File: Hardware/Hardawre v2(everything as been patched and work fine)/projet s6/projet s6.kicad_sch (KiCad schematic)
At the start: 23 parts, among them SW5 RSTBTN, SW6 Int, SW7 boot, U1 STM32L432KCUx, U2 LTC4065AEDC, U3 LDLN022PU33R

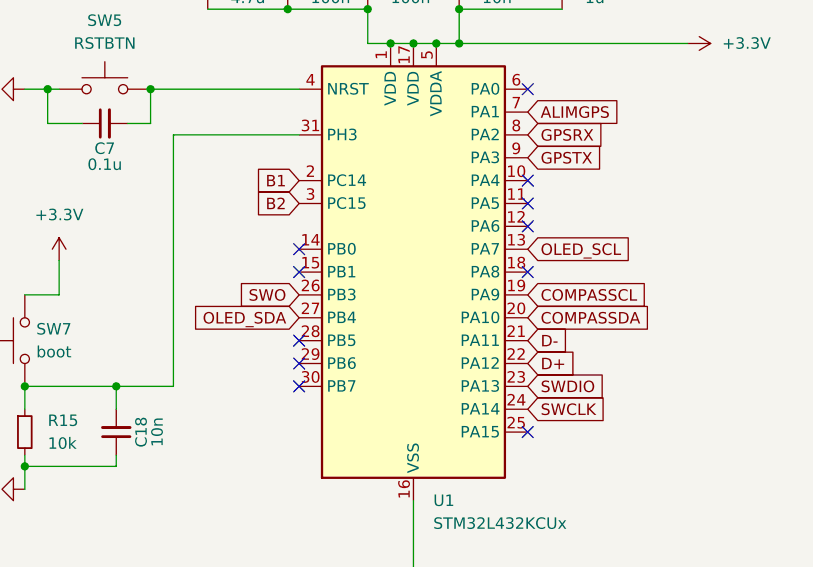
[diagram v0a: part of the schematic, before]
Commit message: gr
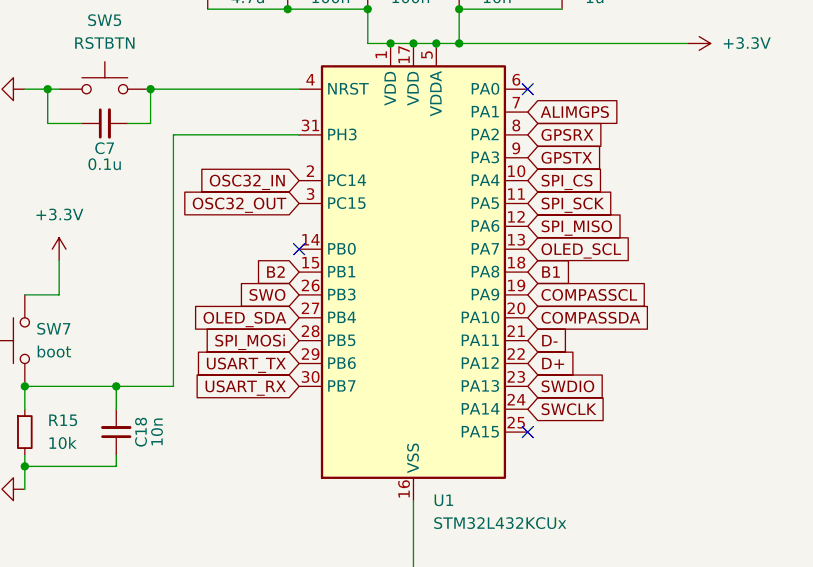
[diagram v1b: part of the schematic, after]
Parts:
- SW5, SW7: footprint SW_KXT3:SW_KXT3 -> KXT3:SW_KXT3
- SW6: footprint SW_PCM:SW_PCM -> PCM:SW_PCM
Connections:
- net B1: now also U1.18 (PA8); no longer U1.2 (PC14)
- net B2: now also U1.15 (PB1); no longer U1.3 (PC15)
- net SPI_CS: now reaches U1.10 (PA4)
- net SPI_SCK: now reaches U1.11 (PA5)
- net SPI_MISO: now reaches U1.12 (PA6)
- net SPI_MOSi: now reaches U1.28 (PB5)
- net USART_TX: now reaches U1.29 (PB6)
- net USART_RX: now reaches U1.30 (PB7)
- new net OSC32_IN: U1.2 (PC14)
- new net OSC32_OUT: U1.3 (PC15)
- no-connect marks 11 -> 3
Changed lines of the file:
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@@
 	)
 	(no_connect
-		(at 233.68 80.01)
-	)
-	(no_connect
-		(at 208.28 95.25)
-	)
-	(no_connect
-		(at 233.68 85.09)
-	)
-	(no_connect
 		(at 233.68 102.87)
 	)
 	(no_connect
-		(at 233.68 74.93)
-	)
-	(no_connect
 		(at 233.68 64.77)
 	)
 	(no_connect
-		(at 208.28 92.71)
-	)
-	(no_connect
-		(at 208.28 97.79)
-	)
-	(no_connect
 		(at 208.28 82.55)
 	)
-	(no_connect
-		(at 208.28 85.09)
-	)
-	(no_connect
-		(at 233.68 77.47)
-	)
 	(wire
 		(pts
@@
 		)
 	)
+	(global_label "OSC32_OUT"
+		(shape input)
+		(at 208.28 77.47 180)
+		(fields_autoplaced yes)
+		(effects
+			(font
+				(size 1.27 1.27)
+			)
+			(justify right)
+		)
+		(property "Intersheetrefs" "${INTERSHEET_REFS}"
+			(at 194.4696 77.47 0)
+			(effects
+				(font
+					(size 1.27 1.27)
+				)
+				(justify right)
+				(hide yes)
+			)
+		)
+	)
 	(global_label "SWO"
 		(shape input)
@@
 		)
 	)
+	(global_label "OSC32_IN"
+		(shape input)
+		(at 208.28 74.93 180)
+		(fields_autoplaced yes)
+		(effects
+			(font
+				(size 1.27 1.27)
+			)
+			(justify right)
+		)
+		(property "Intersheetrefs" "${INTERSHEET_REFS}"
+			(at 196.1629 74.93 0)
+			(effects
+				(font
+					(size 1.27 1.27)
+				)
+				(justify right)
+				(hide yes)
+			)
+		)
+	)
+	(global_label "SPI_MOSi"
+		(shape input)
+		(at 208.28 92.71 180)
+		(fields_autoplaced yes)
+		(effects
+			(font
+				(size 1.27 1.27)
+			)
+			(justify right)
+		)
+		(property "Intersheetrefs" "${INTERSHEET_REFS}"
+			(at 196.6467 92.71 0)
+			(effects
+				(font
+					(size 1.27 1.27)
+				)
+				(justify right)
+				(hide yes)
+			)
+		)
+	)
 	(global_label "GPSRX"
 		(shape input)
@@
 		)
 	)
+	(global_label "SPI_CS"
+		(shape input)
+		(at 233.68 74.93 0)
+		(fields_autoplaced yes)
+		(effects
+			(font
+				(size 1.27 1.27)
+			)
+			(justify left)
+		)
+		(property "Intersheetrefs" "${INTERSHEET_REFS}"
+			(at 243.1966 74.93 0)
+			(effects
+				(font
+					(size 1.27 1.27)
+				)
+				(justify left)
+				(hide yes)
+			)
+		)
+	)
 	(global_label "COMPASSDA"
 		(shape input)
@@
 		)
 	)
+	(global_label "USART_TX"
+		(shape input)
+		(at 208.28 95.25 180)
+		(fields_autoplaced yes)
+		(effects
+			(font
+				(size 1.27 1.27)
+			)
+			(justify right)
+		)
+		(property "Intersheetrefs" "${INTERSHEET_REFS}"
+			(at 196.2839 95.25 0)
+			(effects
+				(font
+					(size 1.27 1.27)
+				)
+				(justify right)
+				(hide yes)
+			)
+		)
+	)
 	(global_label "vusb"
 		(shape input)
@@
 		)
 	)
-	(global_label "B1"
+	(global_label "B2"
 		(shape input)
-		(at 208.28 74.93 180)
+		(at 208.28 85.09 180)
 		(fields_autoplaced yes)
 		(effects
@@
 		)
 		(property "Intersheetrefs" "${INTERSHEET_REFS}"
-			(at 202.8153 74.93 0)
+			(at 202.8153 85.09 0)
 			(effects
 				(font
@@
 		)
 	)
-	(global_label "B2"
+	(global_label "SPI_MISO"
 		(shape input)
-		(at 208.28 77.47 180)
+		(at 233.68 80.01 0)
+		(fields_autoplaced yes)
+		(effects
+			(font
+				(size 1.27 1.27)
+			)
+			(justify left)
+		)
+		(property "Intersheetrefs" "${INTERSHEET_REFS}"
+			(at 245.3133 80.01 0)
+			(effects
+				(font
+					(size 1.27 1.27)
+				)
+				(justify left)
+				(hide yes)
+			)
+		)
+	)
+	(global_label "B1"
+		(shape input)
+		(at 233.68 85.09 0)
+		(fields_autoplaced yes)
+		(effects
+			(font
+				(size 1.27 1.27)
+			)
+			(justify left)
+		)
+		(property "Intersheetrefs" "${INTERSHEET_REFS}"
+			(at 239.1447 85.09 0)
+			(effects
+				(font
+					(size 1.27 1.27)
+				)
+				(justify left)
+				(hide yes)
+			)
+		)
+	)
+	(global_label "USART_RX"
+		(shape input)
+		(at 208.28 97.79 180)
 		(fields_autoplaced yes)
 		(effects
@@
 		)
 		(property "Intersheetrefs" "${INTERSHEET_REFS}"
-			(at 202.8153 77.47 0)
+			(at 195.9815 97.79 0)
 			(effects
 				(font
@@
 		)
 	)
+	(global_label "SPI_SCK"
+		(shape input)
+		(at 233.68 77.47 0)
+		(fields_autoplaced yes)
+		(effects
+			(font
+				(size 1.27 1.27)
+			)
+			(justify left)
+		)
+		(property "Intersheetrefs" "${INTERSHEET_REFS}"
+			(at 244.4666 77.47 0)
+			(effects
+				(font
+					(size 1.27 1.27)
+				)
+				(justify left)
+				(hide yes)
+			)
+		)
+	)
 	(global_label "COMPASSCL"
 		(shape input)
@@
 			)
 		)
-		(property "Footprint" "SW_KXT3:SW_KXT3"
+		(property "Footprint" "KXT3:SW_KXT3"
 			(at 172.72 92.71 0)
 			(effects
@@
 			)
 		)
-		(property "Footprint" "SW_KXT3:SW_KXT3"
+		(property "Footprint" "KXT3:SW_KXT3"
 			(at 186.69 59.69 0)
 			(effects
@@
 			)
 		)
-		(property "Footprint" "SW_PCM:SW_PCM"
+		(property "Footprint" "PCM:SW_PCM"
 			(at 45.72 40.64 0)
 			(effects
